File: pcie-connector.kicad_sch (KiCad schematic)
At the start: 7 parts, among them J2 PCIe_x16_10146070-113Y0LF-ver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

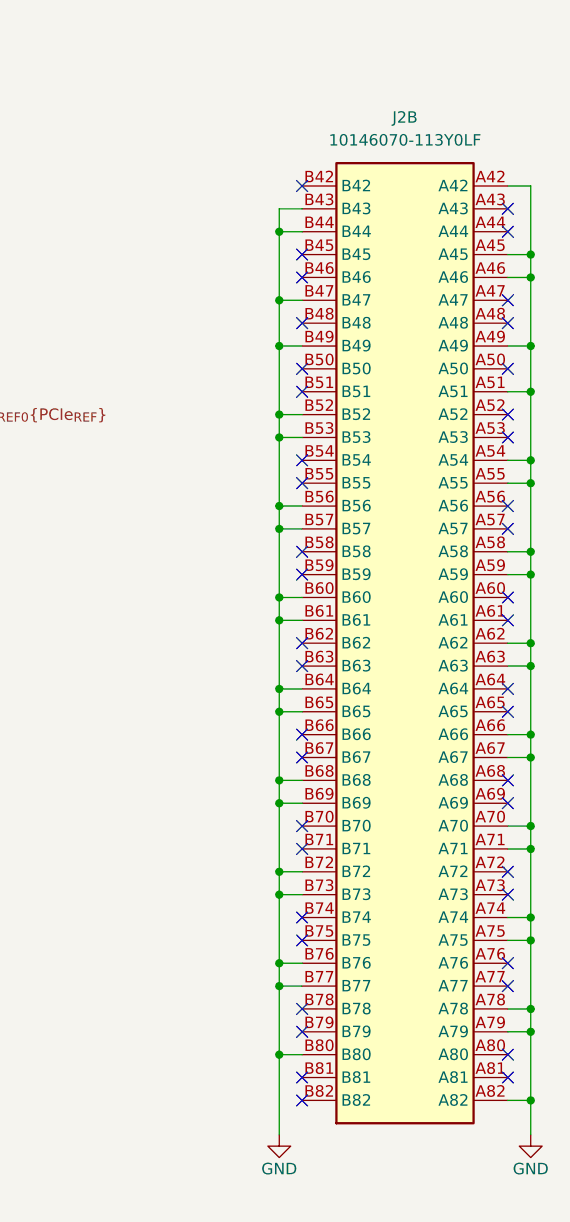
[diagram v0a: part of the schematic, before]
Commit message: [#79262] DRC clean
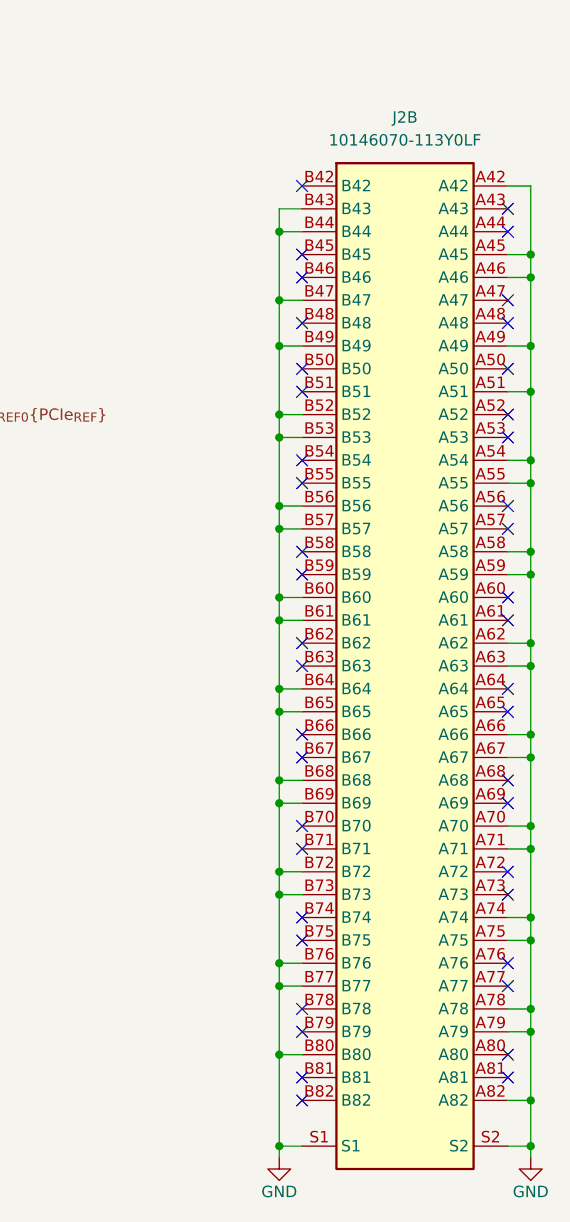
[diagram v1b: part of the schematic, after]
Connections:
- net GND: now also J2.S1, J2.S2
